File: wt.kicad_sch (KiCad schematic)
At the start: 16 parts, among them U4 STM32F407VGTx, Y1 Crystal_8Mhz

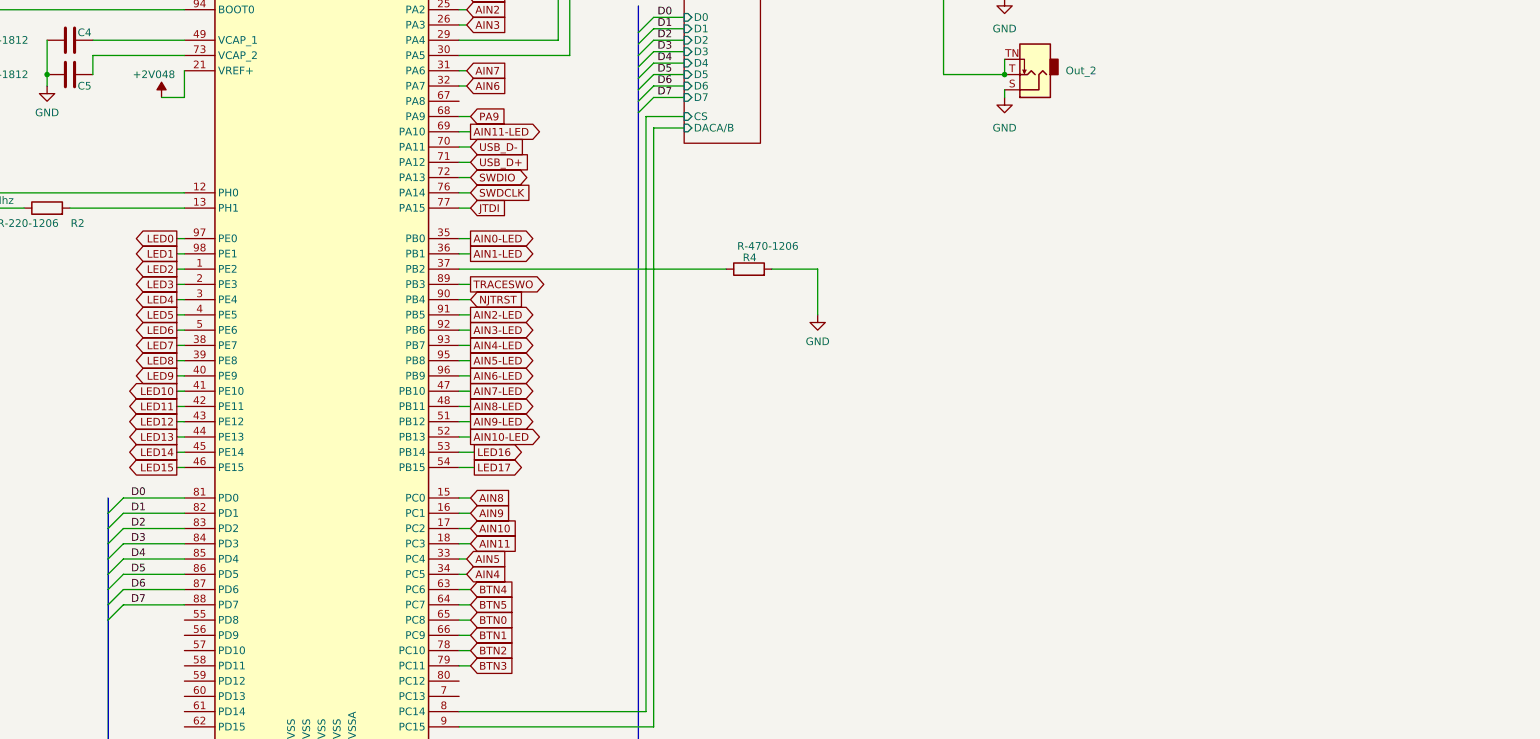
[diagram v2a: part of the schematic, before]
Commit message: yet an other new version with 3 boards
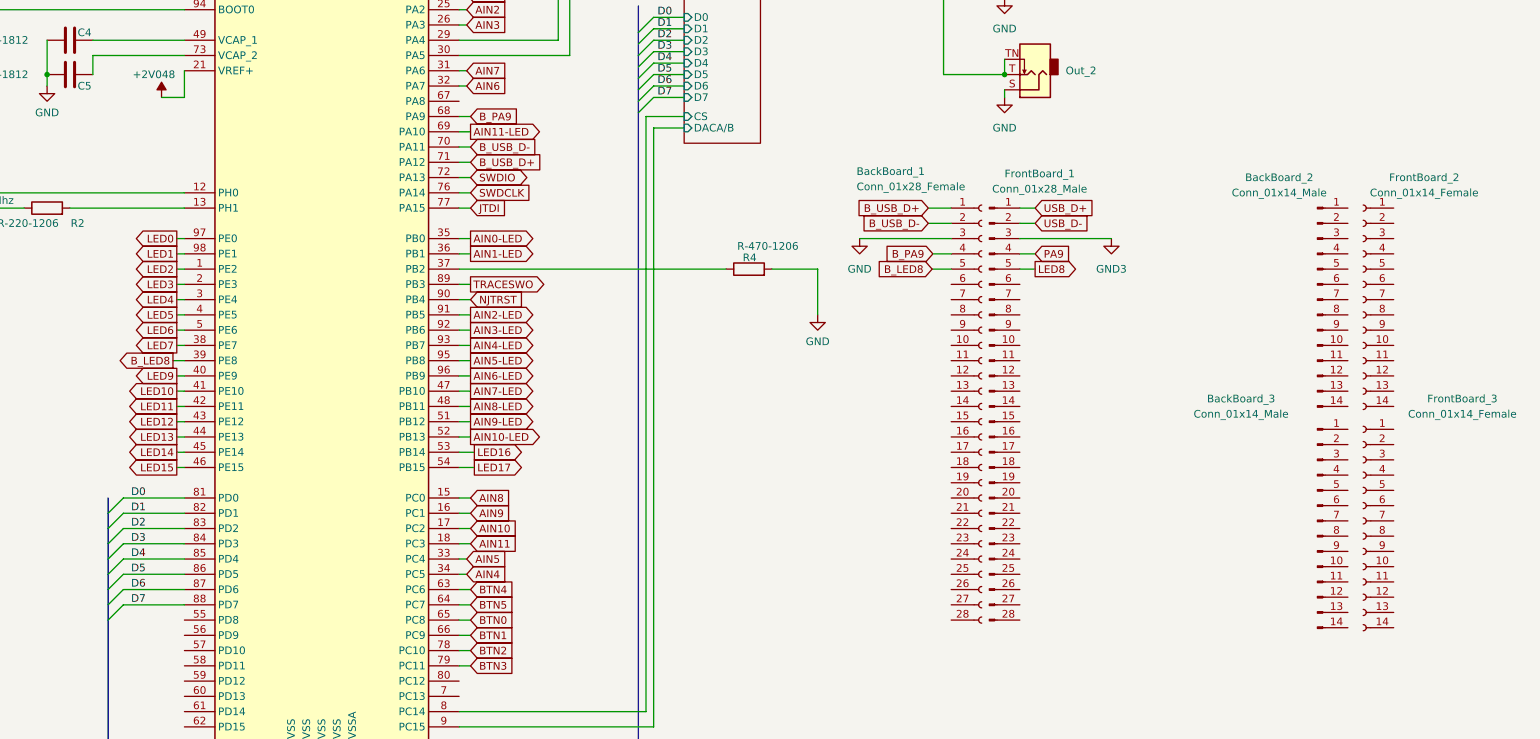
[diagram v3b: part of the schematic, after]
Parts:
- added BackBoard_1: Conn_01x28_Female, Connector_PinSocket_2.54mm:PinSocket_2x14_P2.54mm_Vertical, symbol Connector:Conn_01x28_Female
- added BackBoard_2, BackBoard_3: Conn_01x14_Male, Connector_PinHeader_2.54mm:PinHeader_1x14_P2.54mm_Vertical, symbol Connector:Conn_01x14_Male
- added FrontBoard_1: Conn_01x28_Male, Connector_PinHeader_2.54mm:PinHeader_2x14_P2.54mm_Vertical, symbol Connector:Conn_01x28_Male
- added FrontBoard_2, FrontBoard_3: Conn_01x14_Female, Connector_PinSocket_2.54mm:PinSocket_1x14_P2.54mm_Vertical, symbol Connector:Conn_01x14_Female
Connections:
- net GND: now also BackBoard_1.3 (Pin_3)
- net LED8: now also FrontBoard_1.5 (Pin_5); no longer U4.39 (PE8)
- net PA9: now also FrontBoard_1.4 (Pin_4); no longer U4.68 (PA9)
- net USB_D+: now also FrontBoard_1.1 (Pin_1); no longer U4.71 (PA12)
- net USB_D-: now also FrontBoard_1.2 (Pin_2); no longer U4.70 (PA11)
- new net B_LED8: BackBoard_1.5 (Pin_5), U4.39 (PE8)
- new net B_PA9: BackBoard_1.4 (Pin_4), U4.68 (PA9)
- new net B_USB_D+: BackBoard_1.1 (Pin_1), U4.71 (PA12)
- new net B_USB_D-: BackBoard_1.2 (Pin_2), U4.70 (PA11)
- new net GND3: FrontBoard_1.3 (Pin_3)

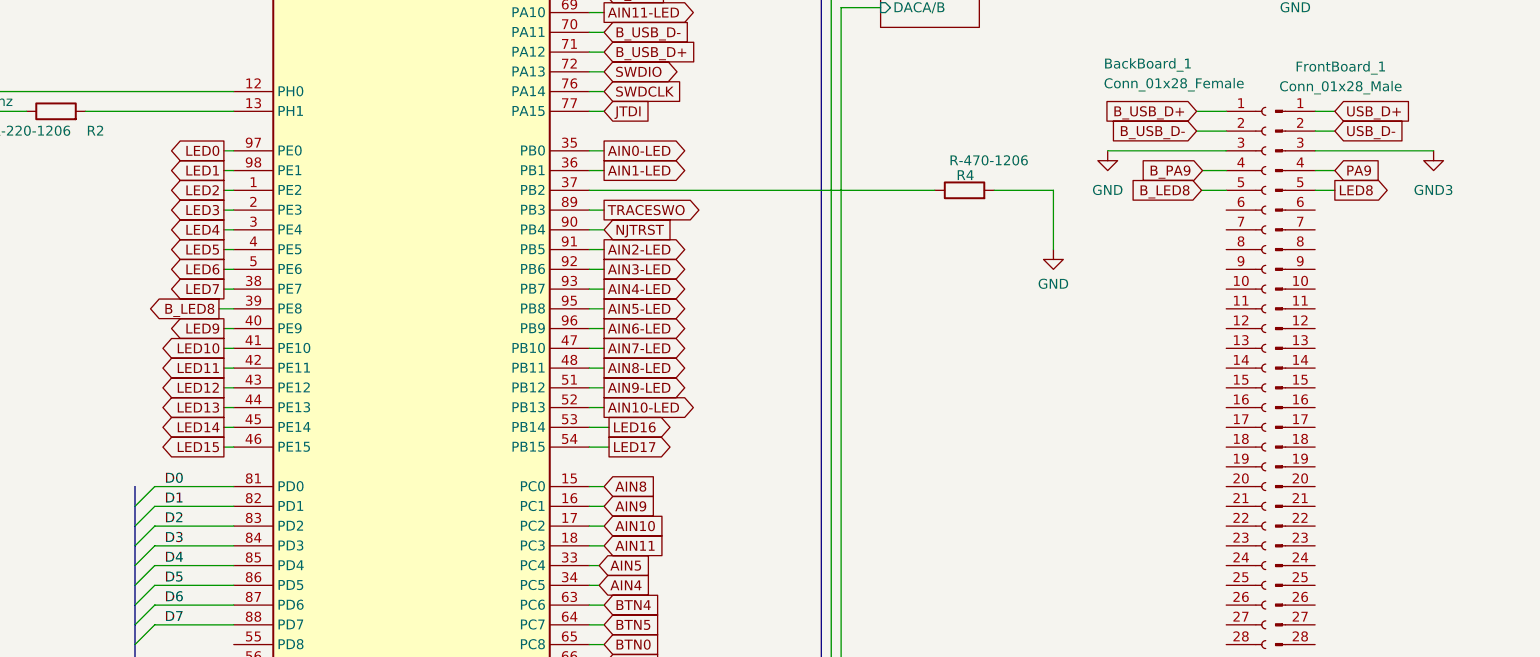
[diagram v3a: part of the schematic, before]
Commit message: this will be a monster
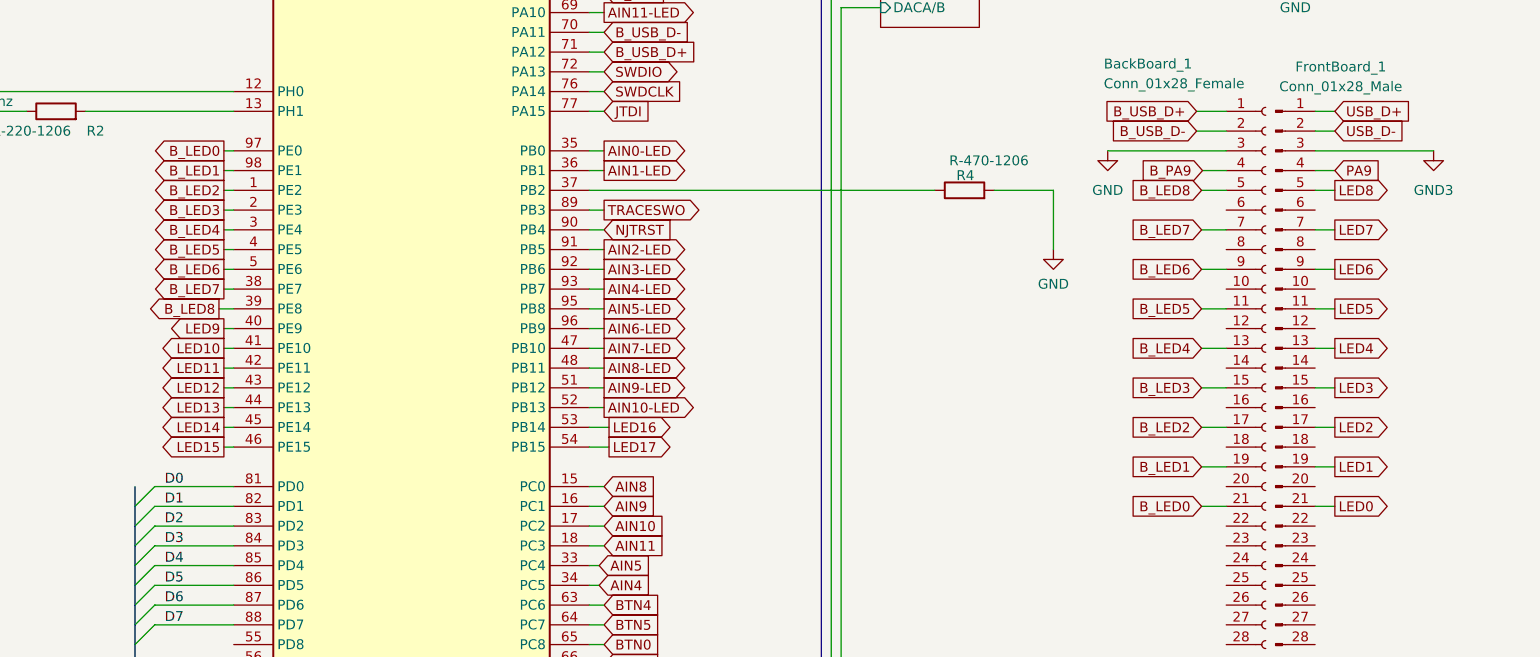
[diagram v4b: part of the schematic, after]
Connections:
- net LED0: now also FrontBoard_1.21 (Pin_21); no longer U4.97 (PE0)
- net LED1: now also FrontBoard_1.19 (Pin_19); no longer U4.98 (PE1)
- net LED2: now also FrontBoard_1.17 (Pin_17); no longer U4.1 (PE2)
- net LED3: now also FrontBoard_1.15 (Pin_15); no longer U4.2 (PE3)
- net LED4: now also FrontBoard_1.13 (Pin_13); no longer U4.3 (PE4)
- net LED5: now also FrontBoard_1.11 (Pin_11); no longer U4.4 (PE5)
- net LED6: now also FrontBoard_1.9 (Pin_9); no longer U4.5 (PE6)
- net LED7: now also FrontBoard_1.7 (Pin_7); no longer U4.38 (PE7)
- net B_LED5: now reaches BackBoard_1.11 (Pin_11)
- net B_LED5: now also U4.4 (PE5)
- net B_LED4: now reaches BackBoard_1.13 (Pin_13)
- net B_LED4: now also U4.3 (PE4)
- net B_LED3: now reaches BackBoard_1.15 (Pin_15)
- net B_LED3: now also U4.2 (PE3)
- net B_LED2: now reaches BackBoard_1.17 (Pin_17)
- net B_LED2: now also U4.1 (PE2)
- net B_LED1: now reaches BackBoard_1.19 (Pin_19)
- net B_LED1: now also U4.98 (PE1)
- net B_LED0: now reaches BackBoard_1.21 (Pin_21)
- net B_LED0: now also U4.97 (PE0)
- net B_LED7: now reaches BackBoard_1.7 (Pin_7)
- net B_LED7: now also U4.38 (PE7)
- net B_LED6: now reaches BackBoard_1.9 (Pin_9)
- net B_LED6: now also U4.5 (PE6)

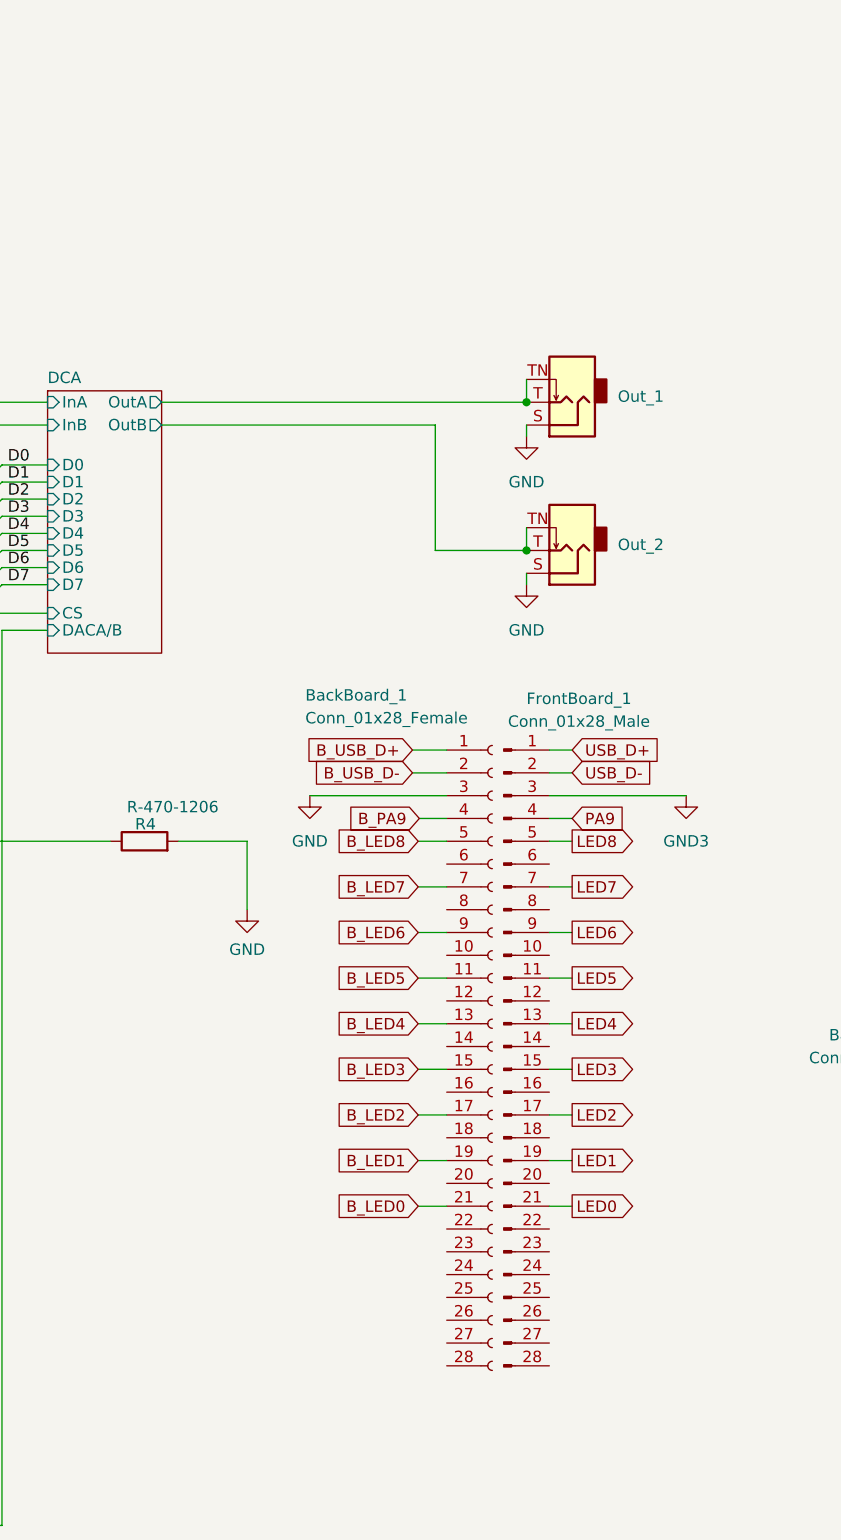
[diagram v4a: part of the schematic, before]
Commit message: working on v3 - so far so good
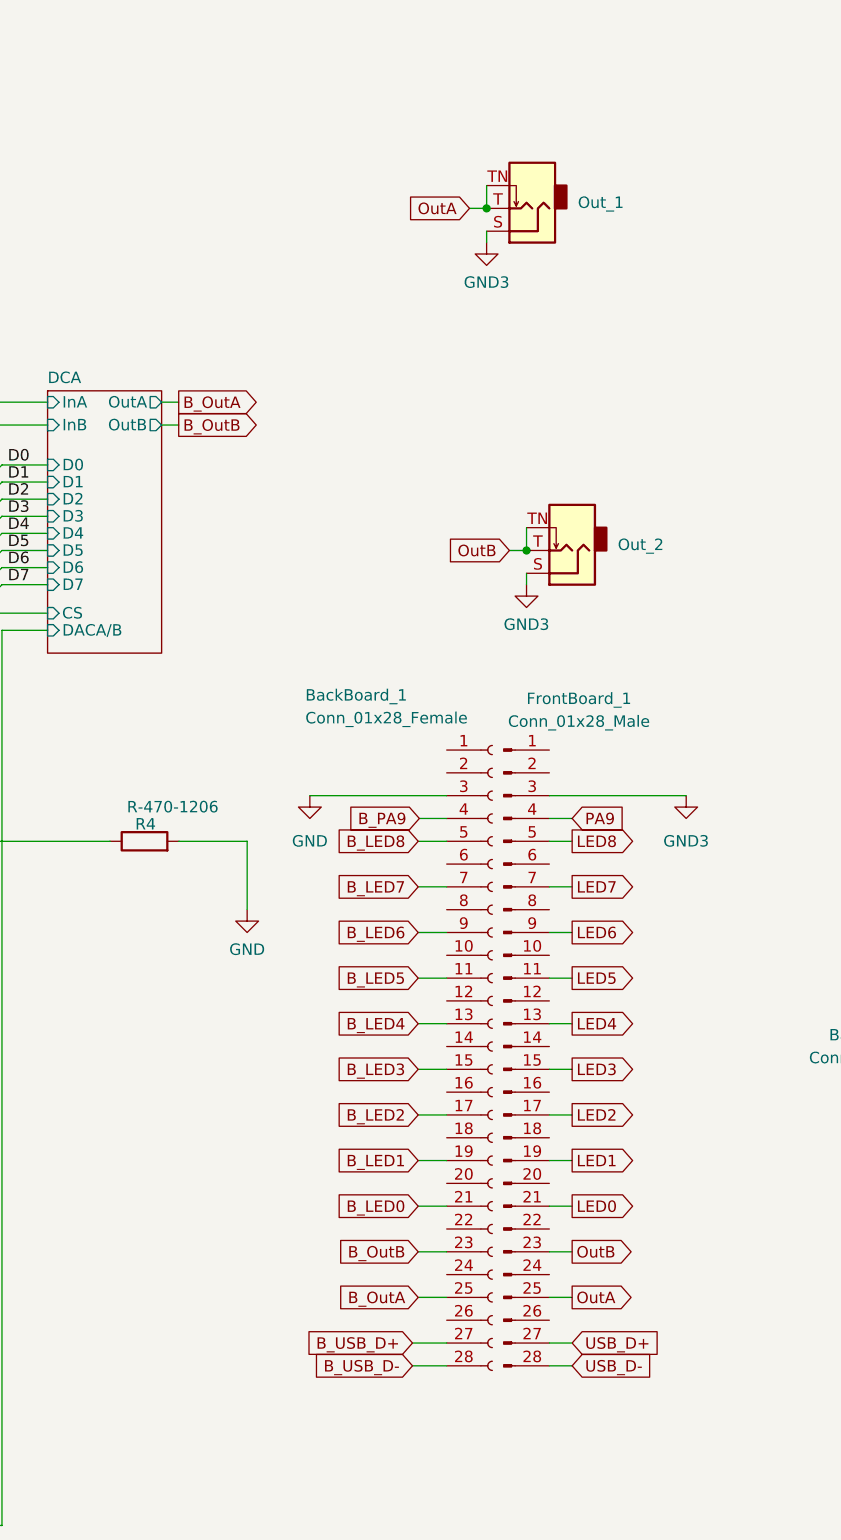
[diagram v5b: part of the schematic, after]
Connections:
- net DCA/OutA is gone; now on net OutA: Out_1.T, Out_1.TN
- net DCA/OutB is gone; now on net OutB: Out_2.T, Out_2.TN
- net B_USB_D+: now also BackBoard_1.27 (Pin_27); no longer BackBoard_1.1 (Pin_1)
- net B_USB_D-: now also BackBoard_1.28 (Pin_28); no longer BackBoard_1.2 (Pin_2)
- net GND: no longer Out_1.S, Out_2.S
- net GND3: now also Out_1.S, Out_2.S
- net USB_D+: now also FrontBoard_1.27 (Pin_27); no longer FrontBoard_1.1 (Pin_1)
- net USB_D-: now also FrontBoard_1.28 (Pin_28); no longer FrontBoard_1.2 (Pin_2)
- net B_OutB: now reaches BackBoard_1.23 (Pin_23)
- net B_OutA: now reaches BackBoard_1.25 (Pin_25)
- net OutB: now reaches FrontBoard_1.23 (Pin_23)
- net OutA: now reaches FrontBoard_1.25 (Pin_25)
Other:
- moved on the sheet: Out_1
